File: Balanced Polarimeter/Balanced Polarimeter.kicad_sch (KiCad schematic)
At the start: 4 parts, among them Q1 MMPQ3904, Q2 MMPQ3904

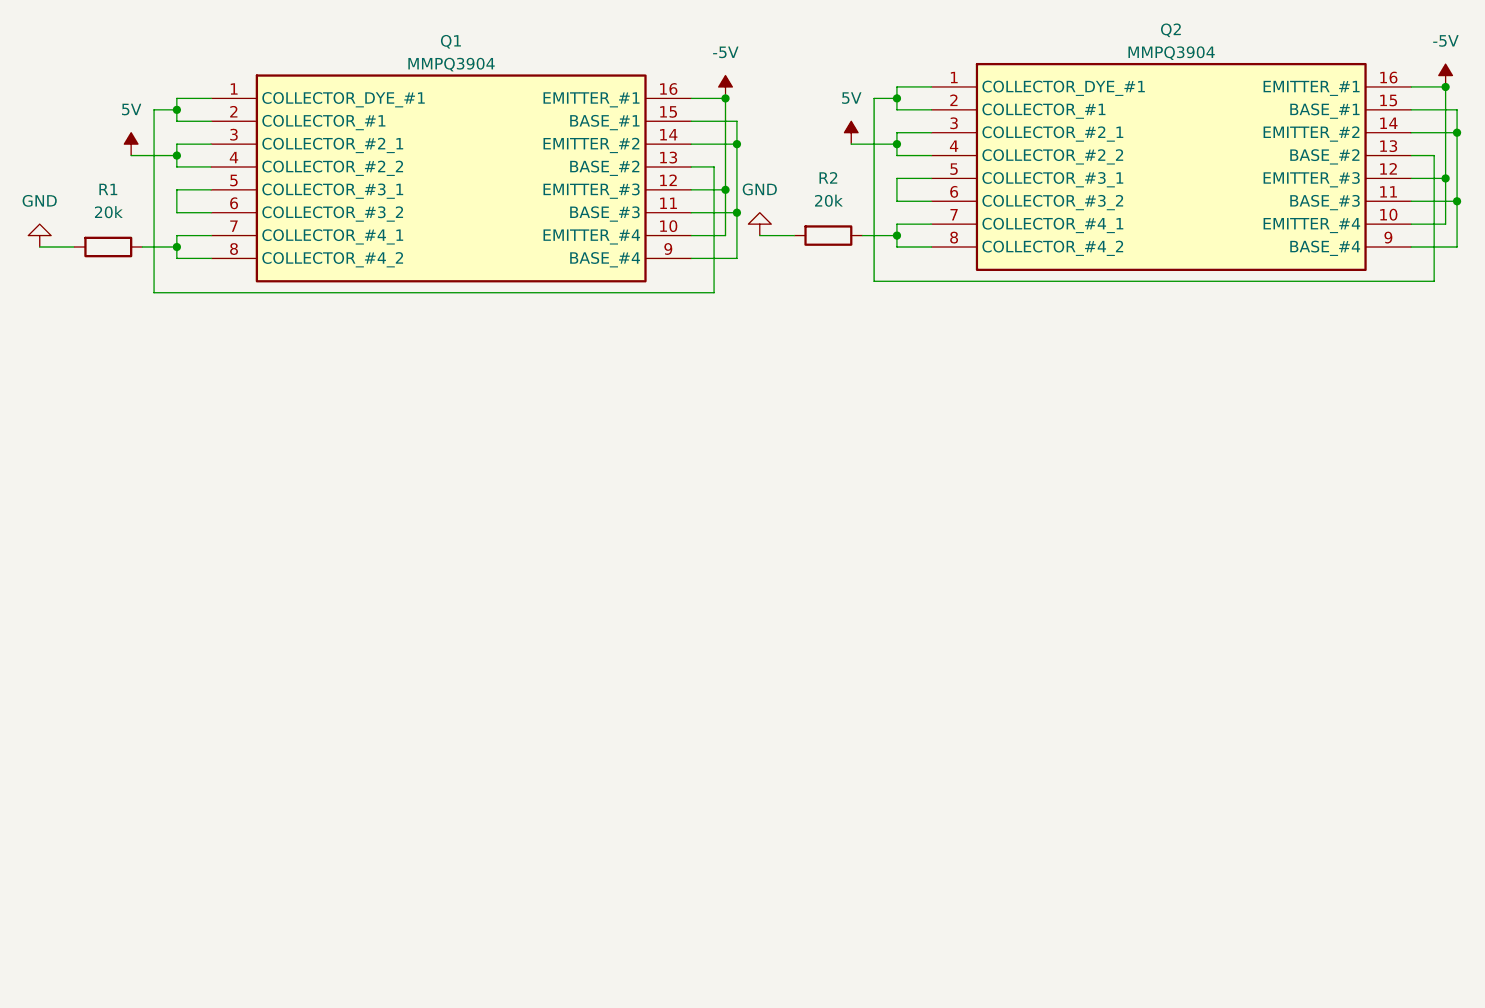
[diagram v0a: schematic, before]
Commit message: Added SS and TA
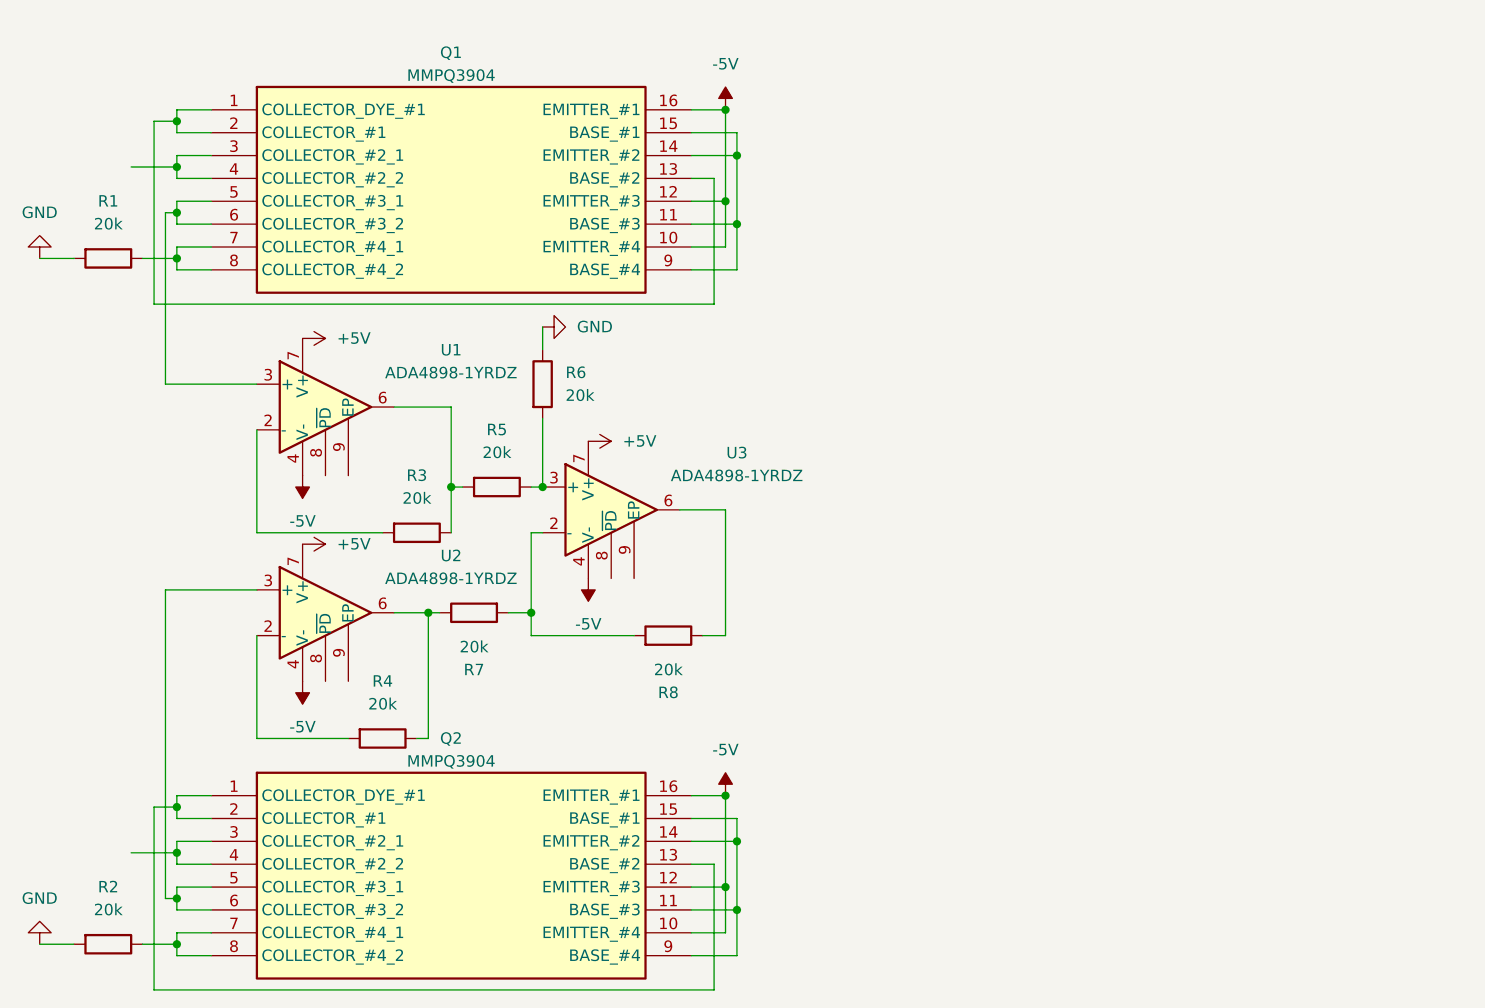
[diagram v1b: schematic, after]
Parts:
- added R3, R4, R5, R6, R7, R8: 20k, symbol Device:R
- added U1, U2, U3: ADA4898-1YRDZ, Package_SO:SOIC-8-1EP_3.9x4.9mm_P1.27mm_EP2.29x3mm, symbol Amplifier_Operational:ADA4898-1YRDZ
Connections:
- net -5V: now also U1.4 (V-), U2.4 (V-), U3.4 (V-)
- net GND: now also R6.1
- net at Q2.5 (COLLECTOR_#3_1), Q2.6 (COLLECTOR_#3_2): now also U2.3 (+)
- net at Q1.5 (COLLECTOR_#3_1), Q1.6 (COLLECTOR_#3_2): now also U1.3 (+)
- net 5V: no longer names the net of Q2.3 (COLLECTOR_#2_1), Q2.4 (COLLECTOR_#2_2)
- net 5V: no longer Q1.3 (COLLECTOR_#2_1), Q1.4 (COLLECTOR_#2_2)
- new net: R4.1, R7.1, U2.6
- new net: R7.2, R8.2, U3.2 (-)
- new net: R5.1, R6.2, U3.3 (+)
- new net: R3.1, R5.2, U1.6
- new net: R4.2, U2.2 (-)
- new net: R8.1, U3.6
- new net: Q1.3 (COLLECTOR_#2_1), Q1.4 (COLLECTOR_#2_2)
- new net: R3.2, U1.2 (-)
- new net +5V: U1.7 (V+), U2.7 (V+), U3.7 (V+)
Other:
- moved on the sheet: Q1, R1
